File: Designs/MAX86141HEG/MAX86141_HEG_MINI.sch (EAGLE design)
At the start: 18 parts, among them U1 MAX86141ENP+T, U3 TXBN0304RUTR, U4 LP5907MFX-3.3/NOPB

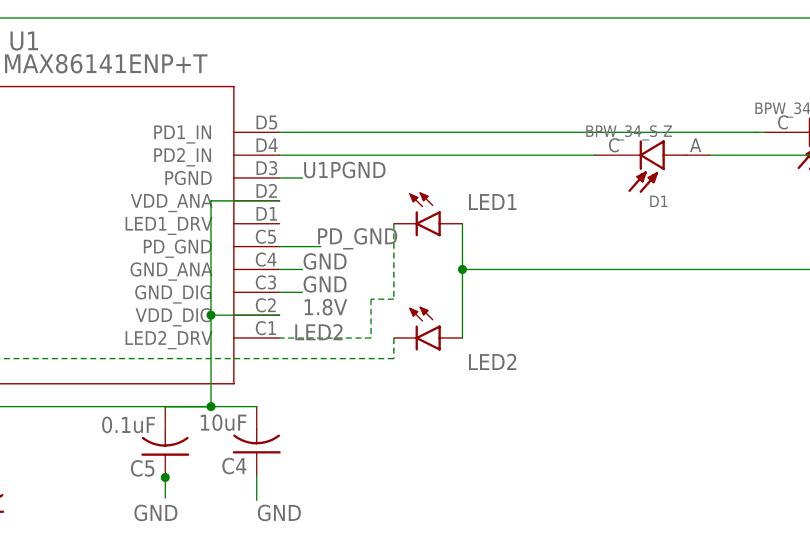
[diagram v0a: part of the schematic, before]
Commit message: updates/another fix for boot routine
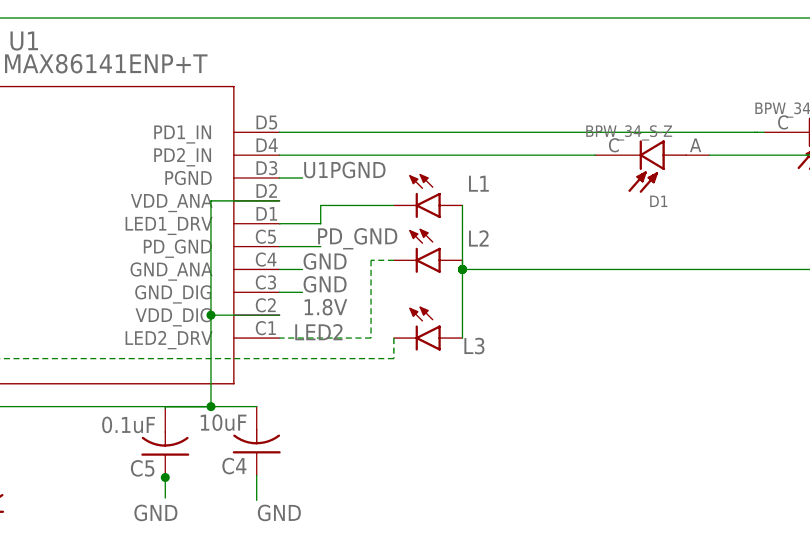
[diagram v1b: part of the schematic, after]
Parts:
- removed LED1: (no value), led:LEDCHIPLED_1206
- added L1, L2: (no value), led:LEDCHIPLED_1206
- renumbered LED2 to L3
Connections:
- new net LED1: L1.C, U1.LED1_DRV
- net 3.3V: now also L1.A, L2.A; no longer LED1.A
- net LED2: now also L2.C; no longer LED1.C
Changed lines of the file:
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@@
 <parts>
 <part name="U1" library="MAX86141" deviceset="MAX86141ENP+T" device=""/>
-<part name="LED1" library="led" library_urn="urn:adsk.eagle:library:259" deviceset="LED" device="CHIPLED_1206" package3d_urn="urn:adsk.eagle:package:15823/2"/>
-<part name="LED2" library="led" library_urn="urn:adsk.eagle:library:259" deviceset="LED" device="CHIPLED_1206" package3d_urn="urn:adsk.eagle:package:15823/2"/>
+<part name="L2" library="led" library_urn="urn:adsk.eagle:library:259" deviceset="LED" device="CHIPLED_1206" package3d_urn="urn:adsk.eagle:package:15823/2"/>
+<part name="L3" library="led" library_urn="urn:adsk.eagle:library:259" deviceset="LED" device="CHIPLED_1206" package3d_urn="urn:adsk.eagle:package:15823/2"/>
 <part name="D1" library="BPW_34_S-Z" deviceset="BPW_34_S-Z" device=""/>
 <part name="D2" library="BPW_34_S-Z" deviceset="BPW_34_S-Z" device=""/>
@@
 <part name="JP2" library="pinhead" library_urn="urn:adsk.eagle:library:325" deviceset="PINHD-1X5" device="" package3d_urn="urn:adsk.eagle:package:22469/2"/>
 <part name="JP3" library="pinhead" library_urn="urn:adsk.eagle:library:325" deviceset="PINHD-1X5" device="" package3d_urn="urn:adsk.eagle:package:22469/2"/>
+<part name="L1" library="led" library_urn="urn:adsk.eagle:library:259" deviceset="LED" device="CHIPLED_1206" package3d_urn="urn:adsk.eagle:package:15823/2"/>
 </parts>
 <sheets>
@@
 <attribute name="VALUE" x="65.7606" y="103.0986" size="2.0828" layer="96" ratio="6" rot="SR0"/>
 </instance>
-<instance part="LED1" gate="G$1" x="114.3" y="86.36" smashed="yes" rot="R270">
-<attribute name="NAME" x="117.348" y="87.884" size="1.778" layer="95"/>
-<attribute name="VALUE" x="109.728" y="80.645" size="1.778" layer="96"/>
-</instance>
-<instance part="LED2" gate="G$1" x="114.3" y="73.66" smashed="yes" rot="R270">
-<attribute name="NAME" x="117.348" y="70.104" size="1.778" layer="95"/>
+<instance part="L2" gate="G$1" x="114.3" y="82.296" smashed="yes" rot="R270">
+<attribute name="NAME" x="117.348" y="83.82" size="1.778" layer="95"/>
+<attribute name="VALUE" x="109.728" y="76.581" size="1.778" layer="96"/>
+</instance>
+<instance part="L3" gate="G$1" x="114.3" y="73.66" smashed="yes" rot="R270">
+<attribute name="NAME" x="116.84" y="71.882" size="1.778" layer="95"/>
 <attribute name="VALUE" x="109.728" y="67.945" size="1.778" layer="96"/>
 </instance>
@@
 <attribute name="NAME" x="-26.67" y="61.849" size="1.778" layer="95" rot="R180"/>
 <attribute name="VALUE" x="-26.67" y="80.264" size="1.778" layer="96" rot="R180"/>
+</instance>
+<instance part="L1" gate="G$1" x="114.3" y="88.392" smashed="yes" rot="R270">
+<attribute name="NAME" x="117.348" y="89.916" size="1.778" layer="95"/>
+<attribute name="VALUE" x="109.728" y="82.677" size="1.778" layer="96"/>
 </instance>
 </instances>
@@
 <wire x1="1.27" y1="81.534" x2="1.27" y2="76.708" width="0.1524" layer="91" style="shortdash"/>
 <junction x="1.27" y="81.534"/>
-<pinref part="LED1" gate="G$1" pin="A"/>
-<wire x1="116.84" y1="86.36" x2="116.84" y2="81.28" width="0.1524" layer="91"/>
+<pinref part="L2" gate="G$1" pin="A"/>
+<wire x1="116.84" y1="82.296" x2="116.84" y2="81.28" width="0.1524" layer="91"/>
+<pinref part="L3" gate="G$1" pin="A"/>
 <wire x1="116.84" y1="81.28" x2="177.8" y2="81.28" width="0.1524" layer="91"/>
-<pinref part="LED2" gate="G$1" pin="A"/>
 <wire x1="177.8" y1="81.28" x2="182.372" y2="81.28" width="0.1524" layer="91"/>
 <wire x1="116.84" y1="73.66" x2="116.84" y2="81.28" width="0.1524" layer="91"/>
@@
 <junction x="23.368" y="65.786"/>
 <wire x1="27.94" y1="55.626" x2="16.764" y2="55.626" width="0.1524" layer="91"/>
+<pinref part="L1" gate="G$1" pin="A"/>
+<wire x1="116.84" y1="88.392" x2="116.84" y2="81.28" width="0.1524" layer="91"/>
+<junction x="116.84" y="81.28"/>
 </segment>
 <segment>
@@
 <net name="LED3" class="0">
 <segment>
-<pinref part="LED2" gate="G$1" pin="C"/>
+<pinref part="L3" gate="G$1" pin="C"/>
 <wire x1="109.22" y1="73.66" x2="109.22" y2="71.374" width="0.1524" layer="91" style="longdash"/>
 <wire x1="109.22" y1="71.374" x2="62.23" y2="71.374" width="0.1524" layer="91" style="longdash"/>
@@
 <net name="LED2" class="0">
 <segment>
-<pinref part="LED1" gate="G$1" pin="C"/>
-<wire x1="109.22" y1="86.36" x2="109.22" y2="77.978" width="0.1524" layer="91" style="longdash"/>
-<wire x1="109.22" y1="77.978" x2="106.68" y2="77.978" width="0.1524" layer="91" style="longdash"/>
+<pinref part="L2" gate="G$1" pin="C"/>
+<wire x1="109.22" y1="82.296" x2="106.68" y2="82.296" width="0.1524" layer="91" style="longdash"/>
 <pinref part="U1" gate="A" pin="LED2_DRV"/>
-<wire x1="106.68" y1="77.978" x2="106.68" y2="73.66" width="0.1524" layer="91" style="longdash"/>
+<wire x1="106.68" y1="82.296" x2="106.68" y2="73.66" width="0.1524" layer="91" style="longdash"/>
 <wire x1="106.68" y1="73.66" x2="96.52" y2="73.66" width="0.1524" layer="91" style="longdash"/>
 <label x="98.044" y="73.406" size="1.778" layer="95"/>
 </segment>
 </net>
+<net name="LED1" class="0">
+<segment>
+<pinref part="U1" gate="A" pin="LED1_DRV"/>
+<wire x1="96.52" y1="86.36" x2="101.092" y2="86.36" width="0.1524" layer="91"/>
+<wire x1="101.092" y1="86.36" x2="101.092" y2="88.392" width="0.1524" layer="91"/>
+<pinref part="L1" gate="G$1" pin="C"/>
+<wire x1="101.092" y1="88.392" x2="109.22" y2="88.392" width="0.1524" layer="91"/>
+</segment>
+</net>

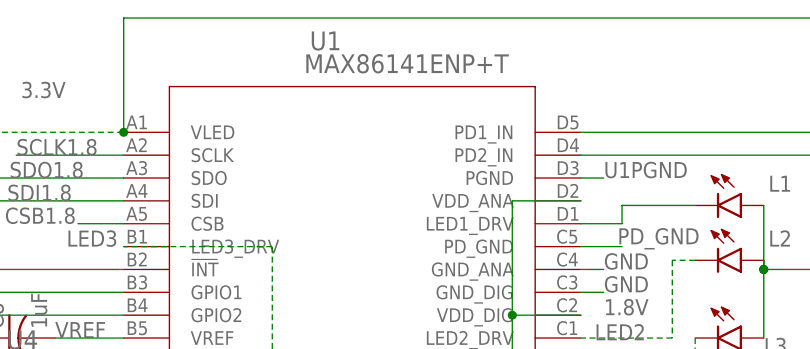
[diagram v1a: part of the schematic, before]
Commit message: quality improvements to design (hopefully)
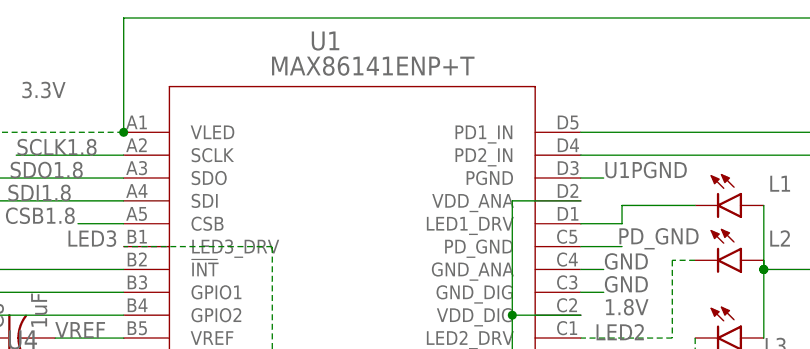
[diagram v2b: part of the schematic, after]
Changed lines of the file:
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@@
 <?xml version="1.0" encoding="utf-8"?>
 <!DOCTYPE eagle SYSTEM "eagle.dtd">
-<eagle version="9.5.1">
+<eagle version="9.6.2">
 <drawing>
 <settings>
@@
 <grid distance="10" unitdist="mil" unit="mil" style="lines" multiple="1" display="no" altdistance="0.01" altunitdist="inch" altunit="inch"/>
 <layers>
-<layer number="1" name="Top" color="4" fill="1" visible="no" active="no"/>
-<layer number="2" name="Route2" color="1" fill="3" visible="no" active="no"/>
-<layer number="3" name="Route3" color="4" fill="3" visible="no" active="no"/>
-<layer number="4" name="Route4" color="1" fill="4" visible="no" active="no"/>
-<layer number="5" name="Route5" color="4" fill="4" visible="no" active="no"/>
-<layer number="6" name="Route6" color="1" fill="8" visible="no" active="no"/>
-<layer number="7" name="Route7" color="4" fill="8" visible="no" active="no"/>
-<layer number="8" name="Route8" color="1" fill="2" visible="no" active="no"/>
-<layer number="9" name="Route9" color="4" fill="2" visible="no" active="no"/>
-<layer number="10" name="Route10" color="1" fill="7" visible="no" active="no"/>
-<layer number="11" name="Route11" color="4" fill="7" visible="no" active="no"/>
-<layer number="12" name="Route12" color="1" fill="5" visible="no" active="no"/>
-<layer number="13" name="Route13" color="4" fill="5" visible="no" active="no"/>
-<layer number="14" name="Route14" color="1" fill="6" visible="no" active="no"/>
-<layer number="15" name="Route15" color="4" fill="6" visible="no" active="no"/>
-<layer number="16" name="Bottom" color="1" fill="1" visible="no" active="no"/>
-<layer number="17" name="Pads" color="2" fill="1" visible="no" active="no"/>
-<layer number="18" name="Vias" color="2" fill="1" visible="no" active="no"/>
-<layer number="19" name="Unrouted" color="6" fill="1" visible="no" active="no"/>
-<layer number="20" name="Dimension" color="24" fill="1" visible="no" active="no"/>
-<layer number="21" name="tPlace" color="7" fill="1" visible="no" active="no"/>
-<layer number="22" name="bPlace" color="7" fill="1" visible="no" active="no"/>
-<layer number="23" name="tOrigins" color="15" fill="1" visible="no" active="no"/>
-<layer number="24" name="bOrigins" color="15" fill="1" visible="no" active="no"/>
-<layer number="25" name="tNames" color="7" fill="1" visible="no" active="no"/>
-<layer number="26" name="bNames" color="7" fill="1" visible="no" active="no"/>
-<layer number="27" name="tValues" color="7" fill="1" visible="no" active="no"/>
-<layer number="28" name="bValues" color="7" fill="1" visible="no" active="no"/>
+<layer number="1" name="Top" color="4" fill="1" visible="yes" active="no"/>
+<layer number="2" name="Route2" color="16" fill="1" visible="yes" active="no"/>
+<layer number="3" name="Route3" color="17" fill="1" visible="yes" active="no"/>
+<layer number="4" name="Route4" color="18" fill="1" visible="yes" active="no"/>
+<layer number="5" name="Route5" color="19" fill="1" visible="yes" active="no"/>
+<layer number="6" name="Route6" color="25" fill="1" visible="yes" active="no"/>
+<layer number="7" name="Route7" color="26" fill="1" visible="yes" active="no"/>
+<layer number="8" name="Route8" color="27" fill="1" visible="yes" active="no"/>
+<layer number="9" name="Route9" color="28" fill="1" visible="yes" active="no"/>
+<layer number="10" name="Route10" color="29" fill="1" visible="yes" active="no"/>
+<layer number="11" name="Route11" color="30" fill="1" visible="yes" active="no"/>
+<layer number="12" name="Route12" color="20" fill="1" visible="yes" active="no"/>
+<layer number="13" name="Route13" color="21" fill="1" visible="yes" active="no"/>
+<layer number="14" name="Route14" color="22" fill="1" visible="yes" active="no"/>
+<layer number="15" name="Route15" color="23" fill="1" visible="yes" active="no"/>
+<layer number="16" name="Bottom" color="1" fill="1" visible="yes" active="no"/>
+<layer number="17" name="Pads" color="2" fill="1" visible="yes" active="no"/>
+<layer number="18" name="Vias" color="2" fill="1" visible="yes" active="no"/>
+<layer number="19" name="Unrouted" color="6" fill="1" visible="yes" active="no"/>
+<layer number="20" name="Dimension" color="24" fill="1" visible="yes" active="no"/>
+<layer number="21" name="tPlace" color="7" fill="1" visible="yes" active="no"/>
+<layer number="22" name="bPlace" color="7" fill="1" visible="yes" active="no"/>
+<layer number="23" name="tOrigins" color="15" fill="1" visible="yes" active="no"/>
+<layer number="24" name="bOrigins" color="15" fill="1" visible="yes" active="no"/>
+<layer number="25" name="tNames" color="7" fill="1" visible="yes" active="no"/>
+<layer number="26" name="bNames" color="7" fill="1" visible="yes" active="no"/>
+<layer number="27" name="tValues" color="7" fill="1" visible="yes" active="no"/>
+<layer number="28" name="bValues" color="7" fill="1" visible="yes" active="no"/>
 <layer number="29" name="tStop" color="7" fill="3" visible="no" active="no"/>
 <layer number="30" name="bStop" color="7" fill="6" visible="no" active="no"/>
@@
 <layer number="35" name="tGlue" color="7" fill="4" visible="no" active="no"/>
 <layer number="36" name="bGlue" color="7" fill="5" visible="no" active="no"/>
-<layer number="37" name="tTest" color="7" fill="1" visible="no" active="no"/>
-<layer number="38" name="bTest" color="7" fill="1" visible="no" active="no"/>
+<layer number="37" name="tTest" color="7" fill="1" visible="yes" active="no"/>
+<layer number="38" name="bTest" color="7" fill="1" visible="yes" active="no"/>
 <layer number="39" name="tKeepout" color="4" fill="11" visible="no" active="no"/>
 <layer number="40" name="bKeepout" color="1" fill="11" visible="no" active="no"/>
@@
 <layer number="44" name="Drills" color="7" fill="1" visible="no" active="no"/>
 <layer number="45" name="Holes" color="7" fill="1" visible="no" active="no"/>
-<layer number="46" name="Milling" color="3" fill="1" visible="no" active="no"/>
-<layer number="47" name="Measures" color="7" fill="1" visible="no" active="no"/>
-<layer number="48" name="Document" color="7" fill="1" visible="no" active="no"/>
-<layer number="49" name="Reference" color="7" fill="1" visible="no" active="no"/>
-<layer number="50" name="dxf" color="7" fill="1" visible="no" active="no"/>
-<layer number="51" name="tDocu" color="7" fill="1" visible="no" active="no"/>
-<layer number="52" name="bDocu" color="7" fill="1" visible="no" active="no"/>
-<layer number="53" name="tGND_GNDA" color="7" fill="9" visible="no" active="no"/>
-<layer number="54" name="bGND_GNDA" color="1" fill="9" visible="no" active="no"/>
-<layer number="56" name="wert" color="7" fill="1" visible="no" active="no"/>
-<layer number="57" name="tCAD" color="7" fill="1" visible="no" active="no"/>
-<layer number="59" name="tCarbon" color="7" fill="1" visible="no" active="no"/>
-<layer number="60" name="bCarbon" color="7" fill="1" visible="no" active="no"/>
+<layer number="46" name="Milling" color="3" fill="1" visible="yes" active="no"/>
+<layer number="47" name="Measures" color="7" fill="1" visible="yes" active="no"/>
+<layer number="48" name="Document" color="7" fill="1" visible="yes" active="no"/>
+<layer number="49" name="Reference" color="7" fill="1" visible="yes" active="no"/>
+<layer number="50" name="dxf" color="7" fill="1" visible="yes" active="no"/>
+<layer number="51" name="tDocu" color="7" fill="1" visible="yes" active="no"/>
+<layer number="52" name="bDocu" color="7" fill="1" visible="yes" active="no"/>
+<layer number="53" name="tGND_GNDA" color="7" fill="9" visible="yes" active="no"/>
+<layer number="54" name="bGND_GNDA" color="1" fill="9" visible="yes" active="no"/>
+<layer number="56" name="wert" color="7" fill="1" visible="yes" active="no"/>
+<layer number="57" name="tCAD" color="7" fill="1" visible="yes" active="no"/>
+<layer number="59" name="tCarbon" color="7" fill="1" visible="yes" active="no"/>
+<layer number="60" name="bCarbon" color="7" fill="1" visible="yes" active="no"/>
 <layer number="88" name="SimResults" color="9" fill="1" visible="yes" active="yes"/>
 <layer number="89" name="SimProbes" color="9" fill="1" visible="yes" active="yes"/>
@@
 <instance part="U1" gate="A" x="43.18" y="96.52" smashed="yes">
 <attribute name="NAME" x="66.3956" y="105.6386" size="2.0828" layer="95" ratio="6" rot="SR0"/>
-<attribute name="VALUE" x="65.7606" y="103.0986" size="2.0828" layer="96" ratio="6" rot="SR0"/>
+<attribute name="VALUE" x="61.9506" y="102.8446" size="2.0828" layer="96" ratio="6" rot="SR0"/>
 </instance>
 <instance part="L2" gate="G$1" x="114.3" y="82.296" smashed="yes" rot="R270">
